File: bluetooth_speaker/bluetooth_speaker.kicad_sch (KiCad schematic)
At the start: 22 parts, among them U1 MAX98357A, U2 XL4015, U3 ESP32-WROOM-32UE

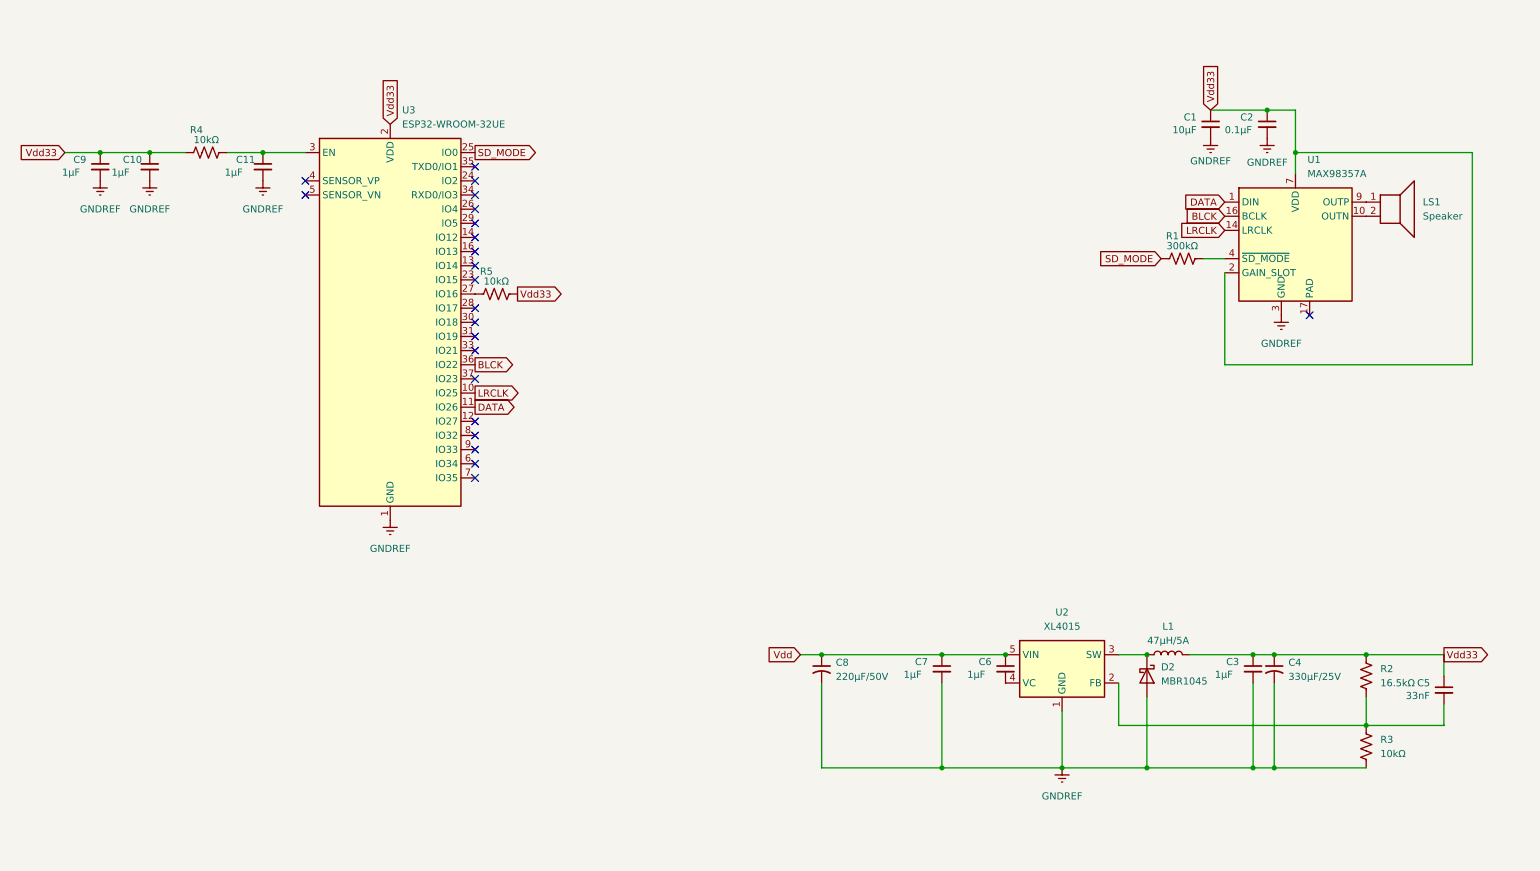
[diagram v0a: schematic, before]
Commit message: Refactor
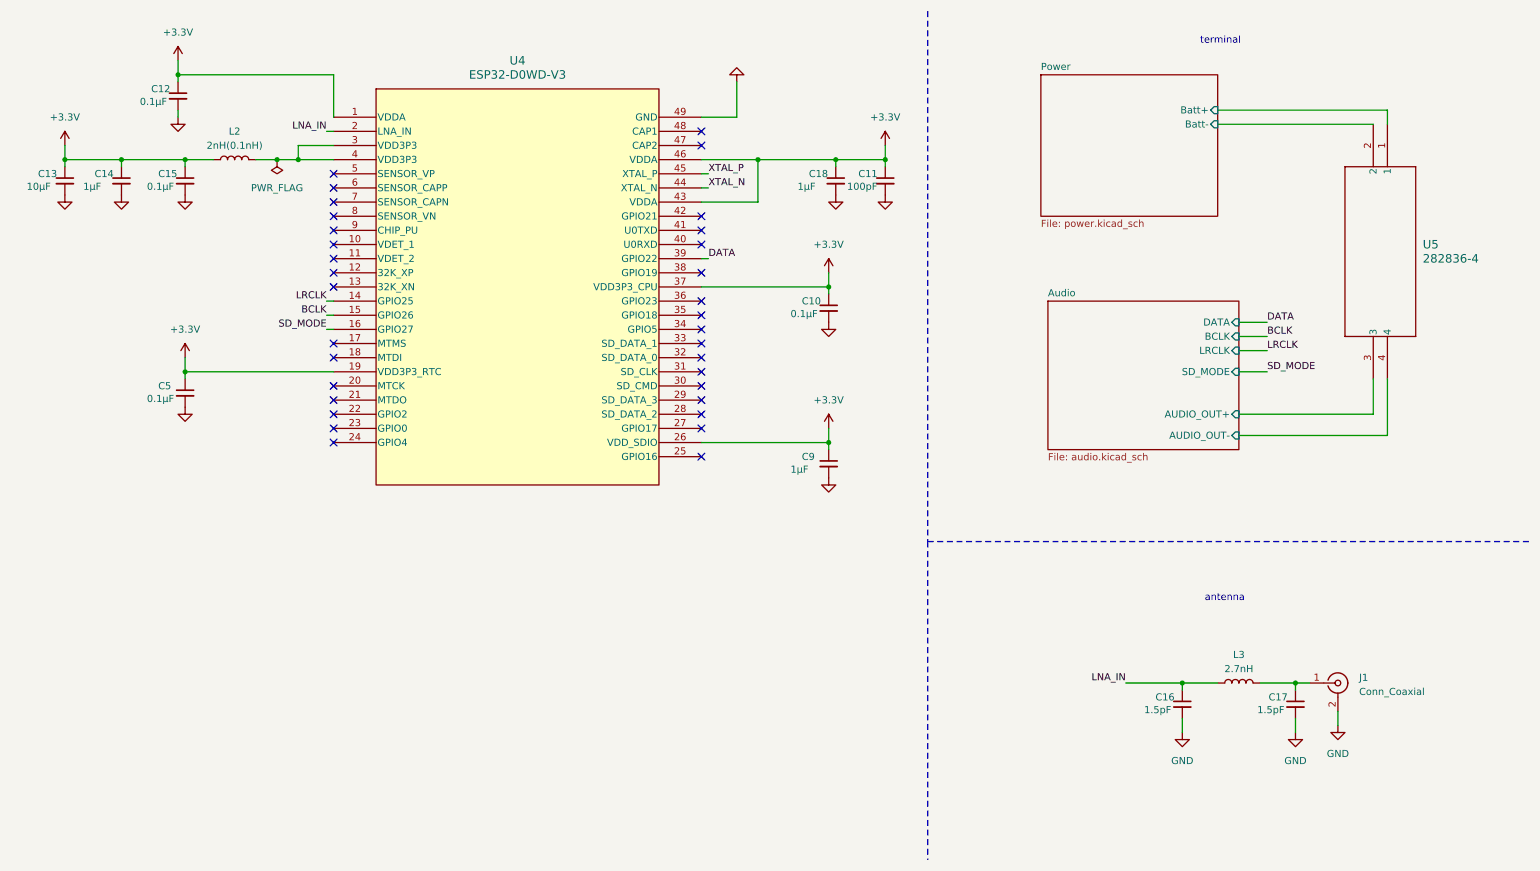
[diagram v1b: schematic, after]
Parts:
- removed C1: 10µF, symbol Device:C_Small
- removed C2: 0.1µF, symbol Device:C_Small
- removed C3, C6, C7: 1µF, symbol Device:C_Small
- removed C4: 330µF/25V, symbol Device:C_Small_US
- removed C8: 220µF/50V, symbol Device:C_Small_US
- removed D2: MBR1045, Package_TO_SOT_THT:TO-220-2_Horizontal_TabDown, symbol Diode:MBR745
- removed L1: 47µH/5A, symbol Device:L
- removed LS1: Speaker, symbol Device:Speaker
- removed R1: 300kΩ, symbol Device:R_US
- removed R2: 16.5kΩ, symbol Device:R_US
- removed R3, R4, R5: 10kΩ, symbol Device:R_US
- removed U1: MAX98357A, Package_DFN_QFN:TQFN-16-1EP_3x3mm_P0.5mm_EP1.23x1.23mm, symbol Audio:MAX98357A
- removed U2: XL4015, Package_TO_SOT_SMD:TO-263-5_TabPin3, symbol Regulator_Switching:XL4015
- removed U3: ESP32-WROOM-32UE, RF_Module:ESP32-WROOM-32UE, symbol RF_Module:ESP32-WROOM-32UE
- added C12, C15: 0.1µF, symbol Device:C_Small
- added C13: 10µF, symbol Device:C_Small
- added C14, C18: 1µF, symbol Device:C_Small
- added C16, C17: 1.5pF, symbol Device:C_Small
- added J1: Conn_Coaxial, symbol Connector:Conn_Coaxial
- added L2: 2nH(0.1nH), symbol Device:L
- added L3: 2.7nH, symbol Device:L
- added U4: ESP32-D0WD-V3, QFN48_ESP32-D0WD-V3_EXP, symbol ESP32-D0WD-V3:ESP32-D0WD-V3
- added U5: 282836-4, 282836-4_TYC, symbol 282836-4:282836-4
- C10: value 1µF -> 0.1µF
- C11: value 1µF -> 100pF
- C5: value 33nF -> 0.1µF
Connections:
- net GNDREF is gone; now on net GND: C10.2, C11.2, C9.2
- net Vdd33 is gone; now on net +3.3V: C10.1, C5.1, C9.1
- net DATA: now also U4.39 (GPIO22)
- net LRCLK: now also U4.14 (GPIO25)
- net SD_MODE: now also U4.16 (GPIO27)
- net GND: now reaches C5.2
- net GND: now also C12.2, C13.2, C14.2, C15.2, C16.2, C17.2, C18.2, J1.2 (Ext), U4.49 (GND)
- net +3.3V: now reaches C11.1
- net +3.3V: now also C12.1, C13.1, C14.1, C15.1, C18.1, L2.1, U4.1 (VDDA), U4.19 (VDD3P3_RTC), U4.26 (VDD_SDIO), U4.37 (VDD3P3_CPU), U4.43 (VDDA), U4.46 (VDDA)
- new net: C17.1, J1.1 (In), L3.2
- new net: L2.2, U4.3 (VDD3P3), U4.4 (VDD3P3)
- new net Audio/AUDIO_OUT+: U5.3
- new net Audio/AUDIO_OUT-: U5.4
- new net BCLK: U4.15 (GPIO26)
- new net LNA_IN: C16.1, L3.1, U4.2 (LNA_IN)
- new net Power/Batt+: U5.1
- new net Power/Batt-: U5.2
- new net XTAL_N: U4.44 (XTAL_N)
- new net XTAL_P: U4.45 (XTAL_P)
- no-connect marks 22 -> 33
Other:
- added sheet Audio (audio.kicad_sch)
- added sheet Power (power.kicad_sch)
- note added: "antenna"
- note added: "terminal"
